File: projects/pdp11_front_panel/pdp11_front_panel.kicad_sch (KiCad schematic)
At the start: 0 parts

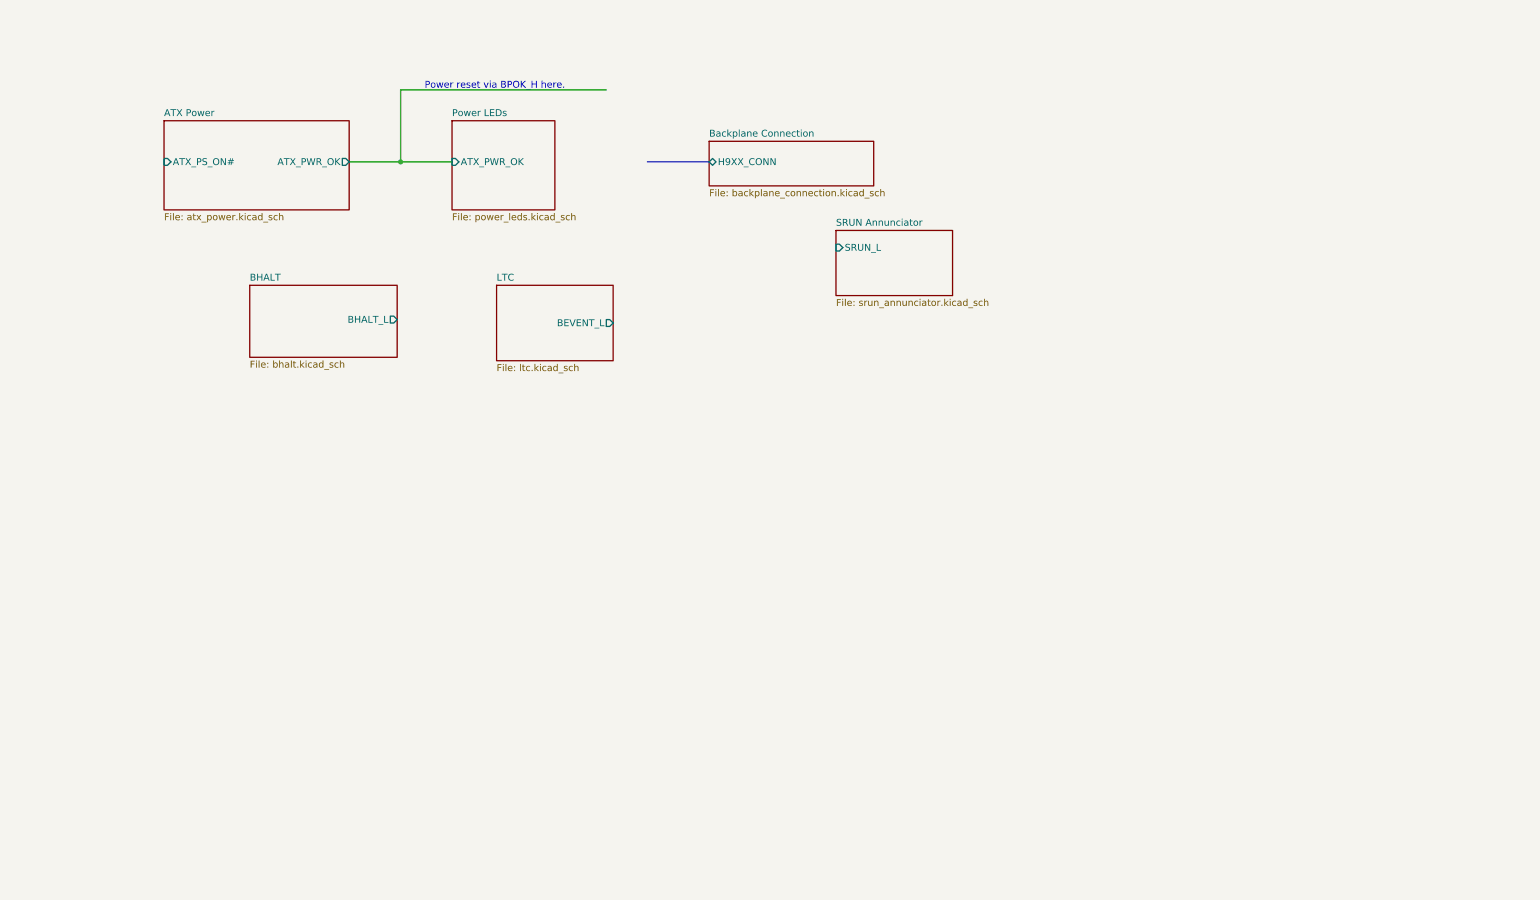
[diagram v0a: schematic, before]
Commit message: .
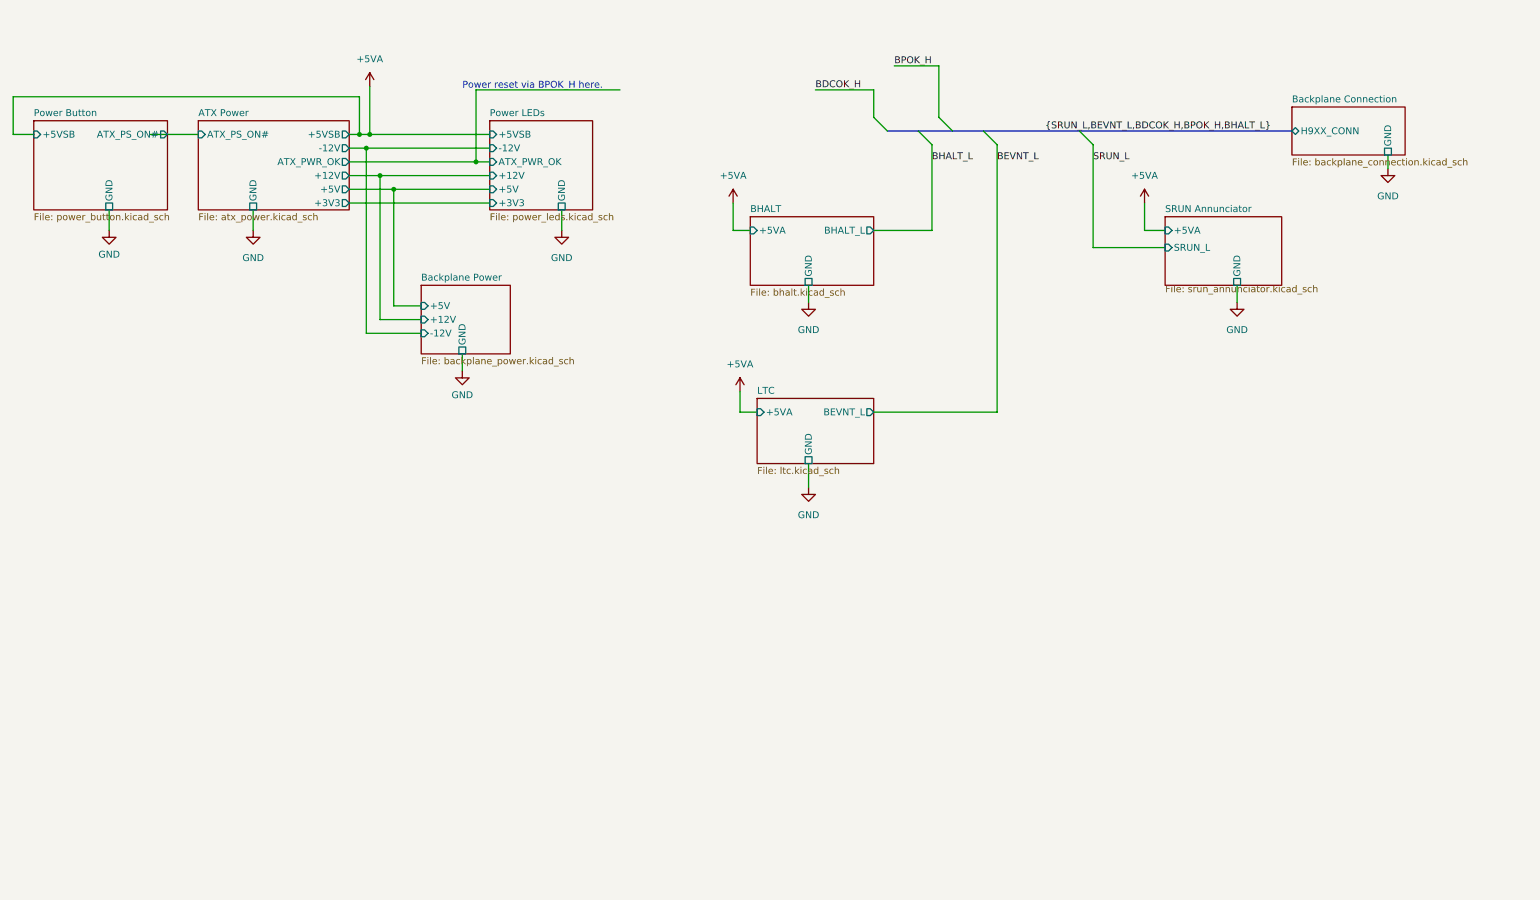
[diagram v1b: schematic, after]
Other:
- added sheet Backplane Power (backplane_power.kicad_sch)
- added sheet Power Button (power_button.kicad_sch)
- sheet ATX Power ports: added +12V, +3V3, +5V, +5VSB, -12V, GND; removed none
- sheet BHALT ports: added +5VA, GND; removed none
- sheet Backplane Connection ports: added GND; removed none
- sheet LTC ports: added +5VA, BEVNT_L, GND; removed BEVENT_L
- sheet Power LEDs ports: added +12V, +3V3, +5V, +5VSB, -12V, GND; removed none
- sheet SRUN Annunciator ports: added +5VA, GND; removed none

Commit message: wip
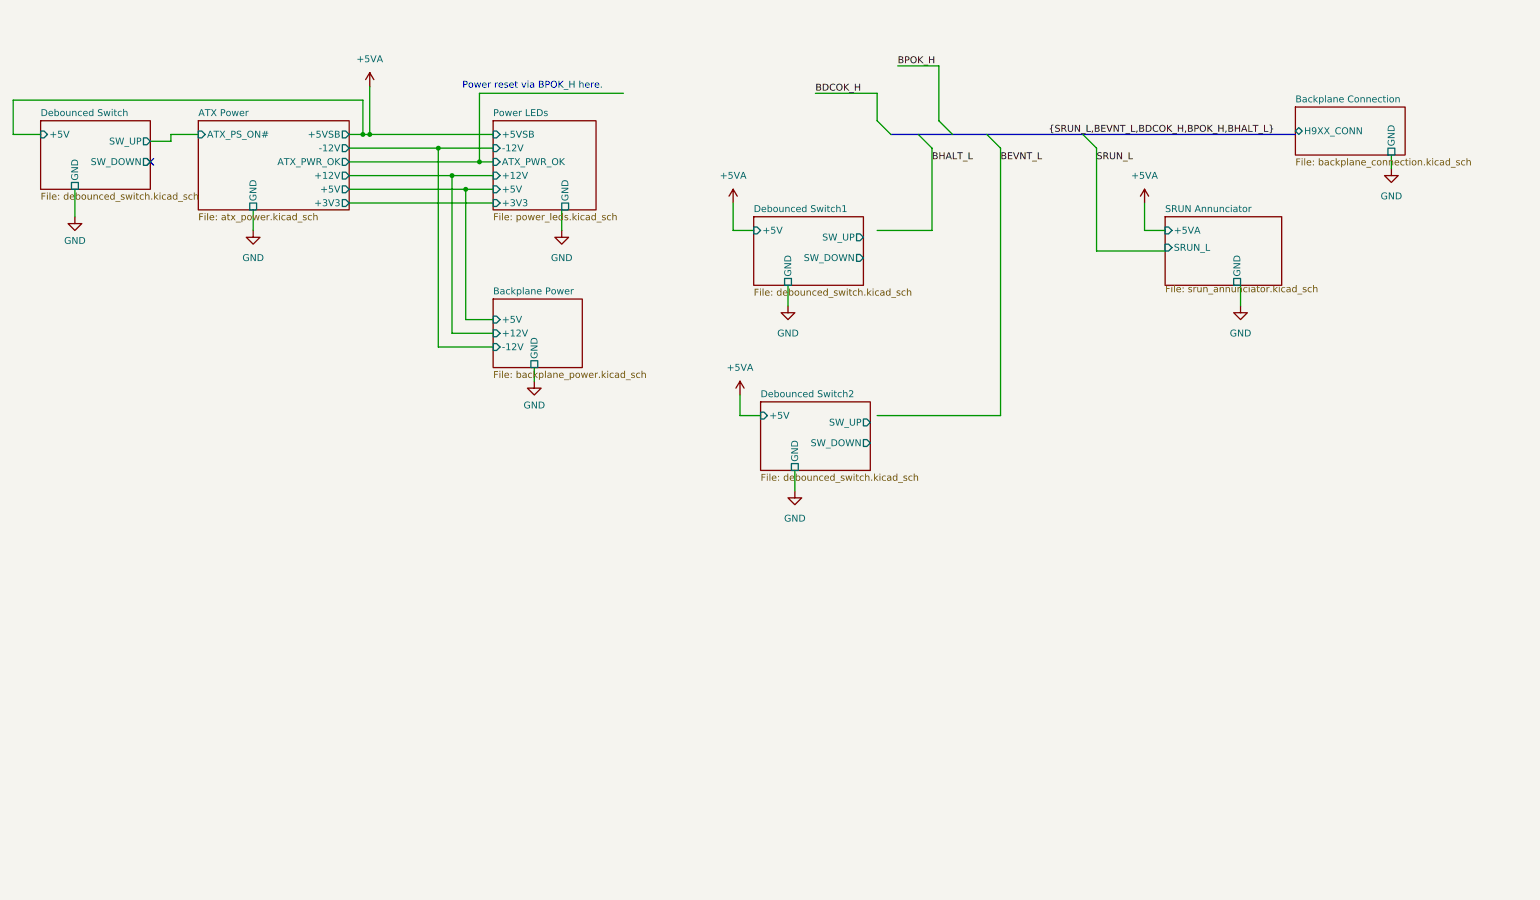
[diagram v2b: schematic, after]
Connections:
- no-connect marks 0 -> 1
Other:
- removed sheet BHALT
- removed sheet LTC
- removed sheet Power Button
- added sheet Debounced Switch (debounced_switch.kicad_sch)
- added sheet Debounced Switch1 (debounced_switch.kicad_sch)
- added sheet Debounced Switch2 (debounced_switch.kicad_sch)

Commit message: wip
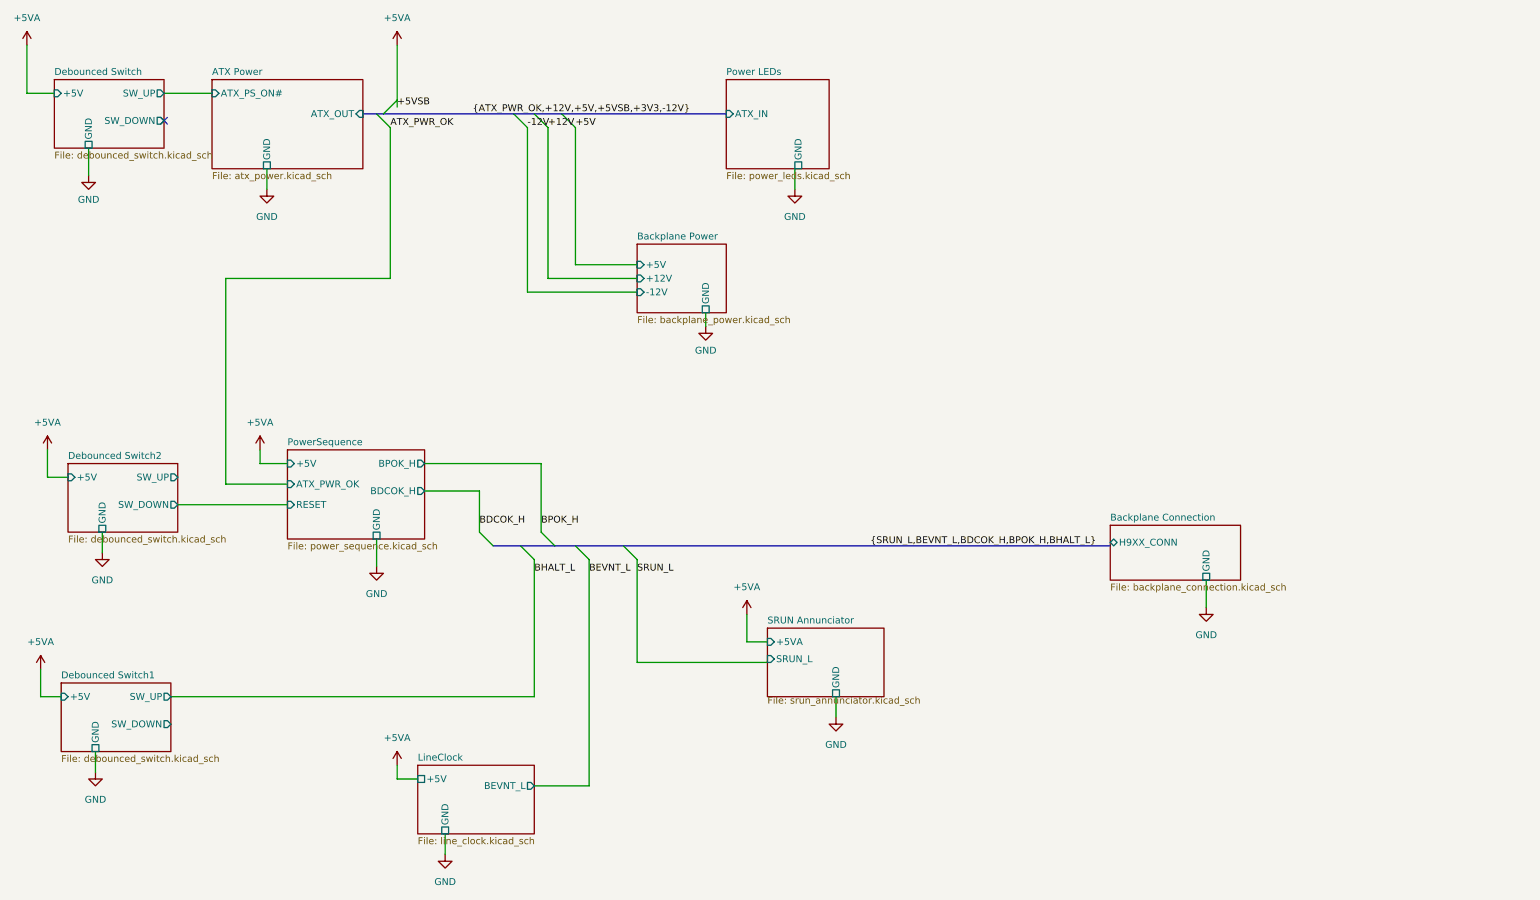
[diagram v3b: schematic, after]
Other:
- added sheet LineClock (line_clock.kicad_sch)
- added sheet PowerSequence (power_sequence.kicad_sch)
- sheet ATX Power ports: added ATX_OUT; removed +12V, +3V3, +5V, +5VSB, -12V, ATX_PWR_OK
- sheet Power LEDs ports: added ATX_IN; removed +12V, +3V3, +5V, +5VSB, -12V, ATX_PWR_OK
- note removed: "Power reset via BPOK_H here."

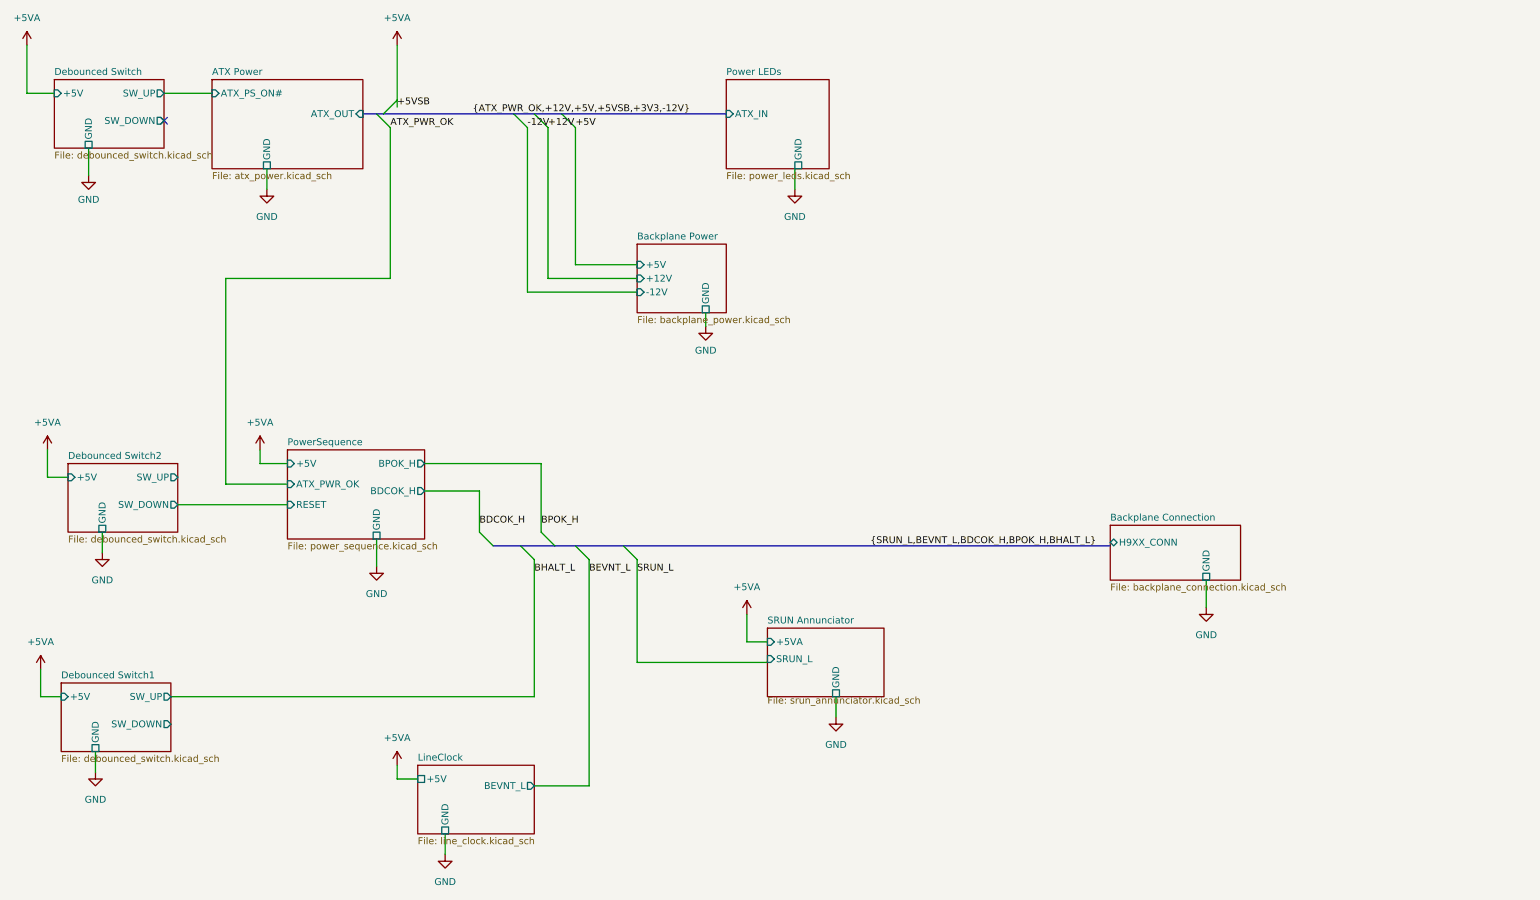
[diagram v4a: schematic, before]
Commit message: wip
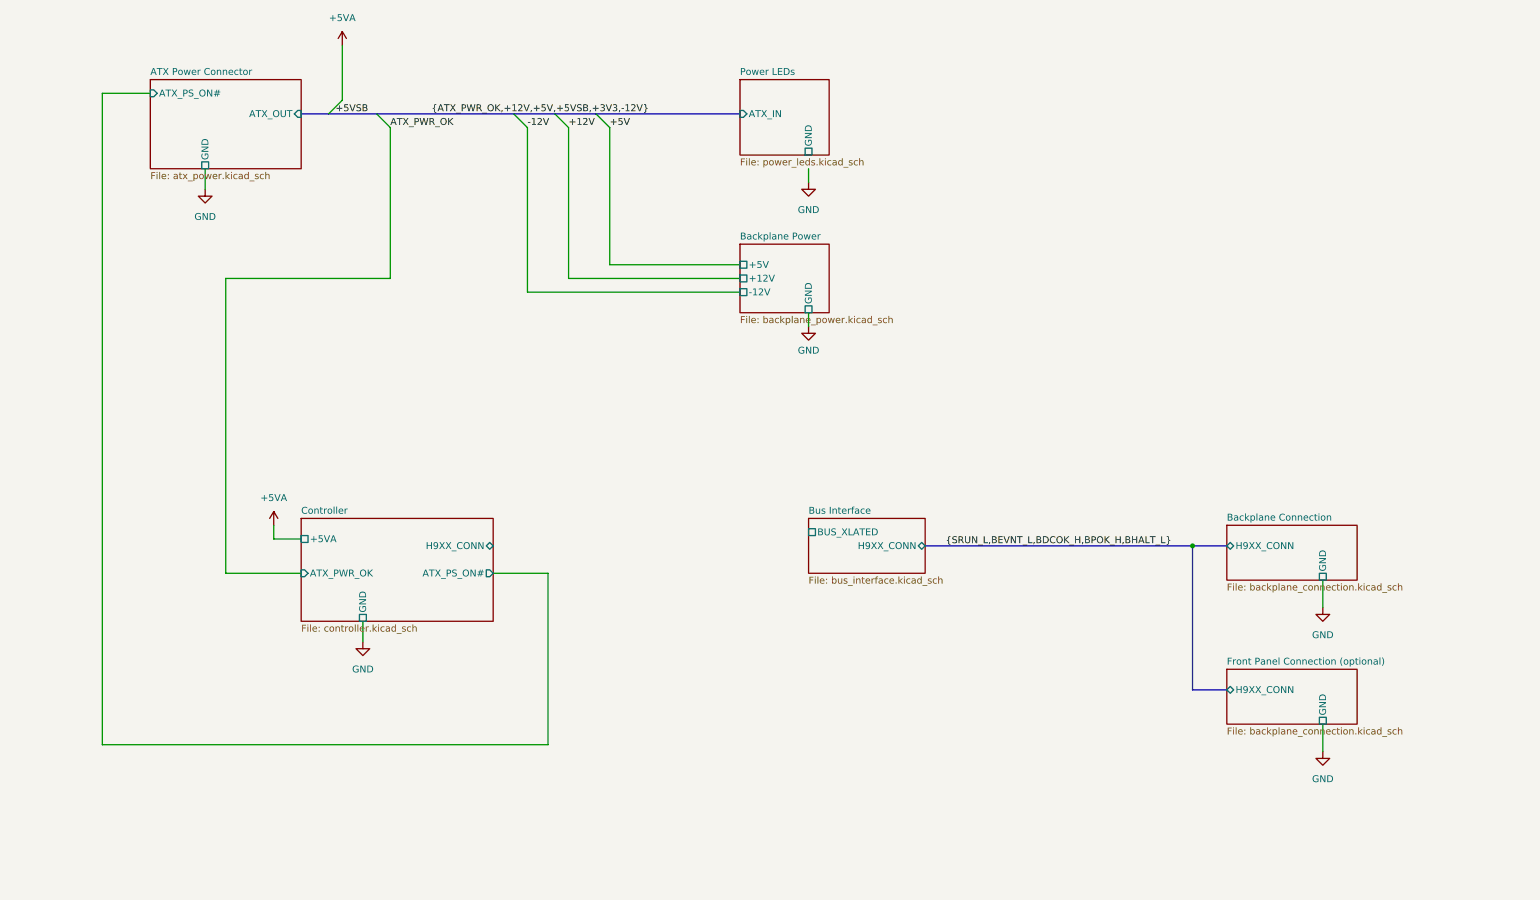
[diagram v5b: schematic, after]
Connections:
- no-connect marks 1 -> 0
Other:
- sheet ATX Power renamed ATX Power Connector
- removed sheet Debounced Switch
- removed sheet Debounced Switch1
- removed sheet Debounced Switch2
- removed sheet LineClock
- removed sheet PowerSequence
- removed sheet SRUN Annunciator
- added sheet Bus Interface (bus_interface.kicad_sch)
- added sheet Controller (controller.kicad_sch)
- added sheet Front Panel Connection (optional) (backplane_connection.kicad_sch)
